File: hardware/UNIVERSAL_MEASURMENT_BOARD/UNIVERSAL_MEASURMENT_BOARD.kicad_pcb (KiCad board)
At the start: 2 copper layers, 68 parts, among them J10 2604-1104, J2 2606-1110_010-000, U1 ADS8863IDGS, U10 TPS54202HDDCR, U12 TPS54202HDDCR, U13 L7805ABD2T-TR, U14 ADM3055EBRIZ-RL, U15 TLV76133KVUR, U16 TLV76133KVUR, U2 LT3471EDD#PBF, U3 CD4067BM96, U4 PGA280AIPW, U5 CD4067BM96, U6 STM32G484RET3, U7 L7812ABD2T-TR, U8 MC7815BDTRKG, Y1 ECS-1612MV

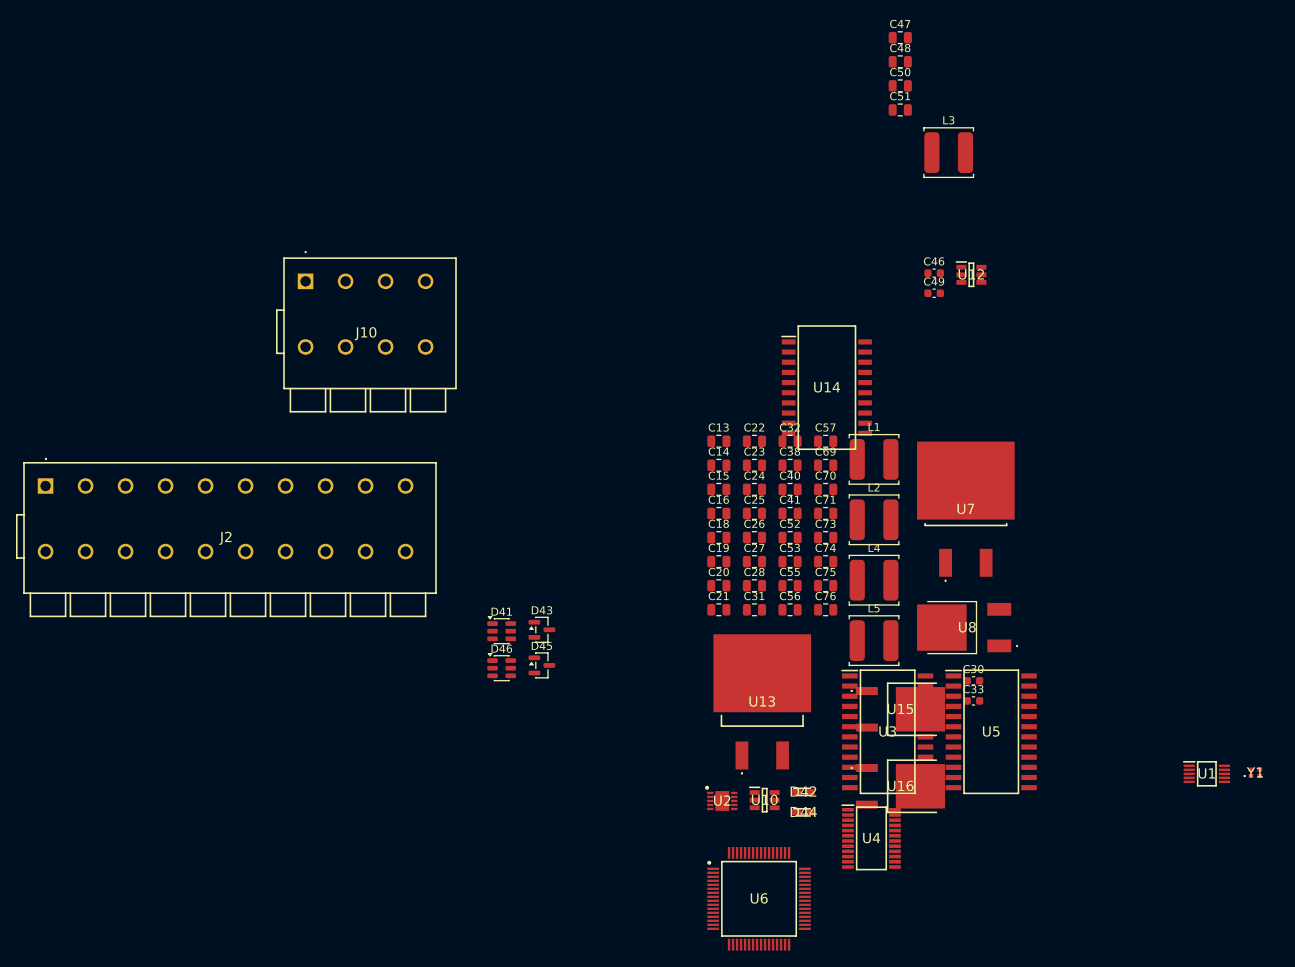
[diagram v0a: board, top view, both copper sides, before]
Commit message: final schematic review corrections
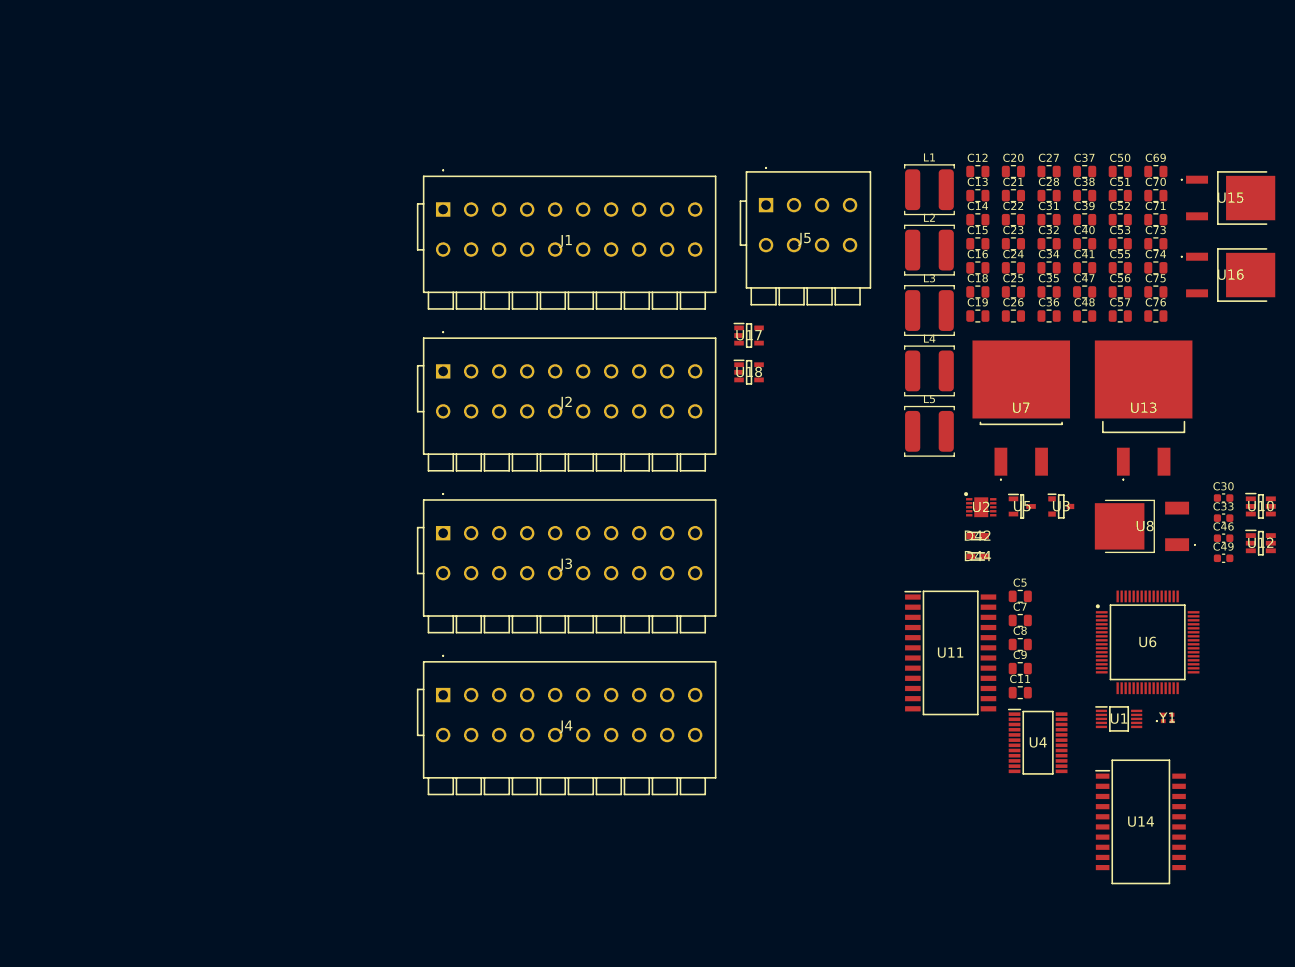
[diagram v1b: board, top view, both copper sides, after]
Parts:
- removed D41, D46: 3.6V/400W, Package_TO_SOT_SMD:SOT-23-6
- removed D43: BZX84C5V6, Package_TO_SOT_SMD:SOT-23
- removed D45: BZX84C3V6-E3-08, Package_TO_SOT_SMD:SOT-23
- removed J10: 2604-1104, 2604-1104:26041104
- added C11: 100nF, Capacitor_SMD:C_0805_2012Metric, F.Cu at (165.4, 110.4)
- added C12: 1uF, Capacitor_SMD:C_0805_2012Metric, F.Cu at (160.2, 45.3)
- added C34: 100nF, Capacitor_SMD:C_0805_2012Metric, F.Cu at (169.1, 57.3)
- added C35: 1uF, Capacitor_SMD:C_0805_2012Metric, F.Cu at (169.1, 60.3)
- added C36: 1uF, Capacitor_SMD:C_0805_2012Metric, F.Cu at (169.1, 63.4)
- added C37: 100nF, Capacitor_SMD:C_0805_2012Metric, F.Cu at (173.5, 45.3)
- added C39: 1uF, Capacitor_SMD:C_0805_2012Metric, F.Cu at (173.5, 51.3)
- added C5: 100nF, Capacitor_SMD:C_0805_2012Metric, F.Cu at (165.4, 98.4)
- added C7: 470nF, Capacitor_SMD:C_0805_2012Metric, F.Cu at (165.4, 101.4)
- added C8: 470nF, Capacitor_SMD:C_0805_2012Metric, F.Cu at (165.4, 104.4)
- added C9: 470nF, Capacitor_SMD:C_0805_2012Metric, F.Cu at (165.4, 107.4)
- added J1: 2606-1110_010-000, 2601-1110:26011110, F.Cu at (93.3, 50.0)
- added J3: 2606-1110_010-000, 2601-1110:26011110, F.Cu at (93.3, 90.5)
- added J4: 2606-1110_010-000, 2601-1110:26011110, F.Cu at (93.3, 110.7)
- added J5: 2604-1104, 2601-1104:26011104, F.Cu at (133.7, 49.5)
- added U11: CD4097BM, CD4097BM:SOIC127P1030X265-24N, F.Cu at (156.8, 105.5)
- added U17: ESDS304DBVR, ESDS304DBVR:SOT95P280X145-5N, F.Cu at (131.6, 65.8)
- added U18: ESDS304DBVR, ESDS304DBVR:SOT95P280X145-5N, F.Cu at (131.6, 70.4)
- J2: footprint 2604-1110:26041110 -> 2601-1110:26011110
- U3: value CD4067BM96 -> MAX6063AEUR+T; footprint CD4067BM96:SOIC127P1030X265-24N -> MAX6063AEUR+T:SOT95P229X119-3N
- U5: value CD4067BM96 -> ISL21010CFH315Z-TK; footprint CD4067BM96:SOIC127P1030X265-24N -> ISL21010CFH315Z-TK:SOT95P237X112-3N
- moved U15 76.1 mm to (191.9, 48.6)
- moved U16 76.1 mm to (191.9, 58.2)
- moved U10 72.1 mm to (195.5, 87.2)
- moved U14 67.0 mm to (180.5, 126.6)
- moved C21 63.5 mm to (164.6, 48.3)
- moved C20 63.5 mm to (164.6, 45.3)
- moved C27 61.1 mm to (169.1, 45.3)
- moved C31 61.1 mm to (169.1, 51.3)
- moved C28 61.1 mm to (169.1, 48.3)
- moved U13 60.2 mm to (180.9, 75.2)
- moved U6 58.2 mm to (181.4, 104.1)
- moved C52 57.3 mm to (177.9, 51.3)
- moved C53 57.3 mm to (177.9, 54.3)
- moved C55 57.3 mm to (177.9, 57.3)
- moved C56 57.3 mm to (177.9, 60.3)
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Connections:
- net +12VA renamed +12V0A
- net +15V renamed +15V0
- net +15VF renamed +15V0F
- net +18V renamed +18V0
- net +7V renamed +7V0
- net -18V renamed -18V0
- net /can/RX renamed /can/CAN_RX
- net /can/TX renamed /can/CAN_TX
- C16 pad 1: +15VA -> +15V0A
- C28 pad 2: -15VA -> -15V0A
- C57 pad 1: +5VA -> +5V0A
- U1 pad 1: Net-(U1-REF) -> +3V0A
- U13 pad 3: +5VA -> +5V0A
- U3 pad 1: Net-(U3-OUT) -> +5V0A
- U3 pad 2: /connectors/A8P -> +3V0A
- U3 pad 3: /connectors/A7P -> GND
- U4 pad 10: Net-(U4-INN1) -> /mux & pga/NS
- U4 pad 11: -15VA -> Net-(U4-VSN)
- U4 pad 13: +3.3VA -> Net-(U4-DVDD)
- U4 pad 3: unconnected-(U4-VOCM-Pad3) -> 1V5A
- U4 pad 4: +3.3VA -> Net-(U4-VSOP)
- U4 pad 6: +15VA -> Net-(U4-VSP)
- U4 pad 9: Net-(U3-OUT) -> /mux & pga/PS
- U5 pad 1: Net-(U4-INN1) -> +3V3A
- U5 pad 2: /connectors/A8N -> +1V5A
- U5 pad 3: /connectors/A7N -> GND
- U6 pad 28: unconnected-(U6-VREF+-Pad28) -> 3V0A
- U6 pad 30: /mcu & adc/UART_RX_PROG -> /connectors/UART_RX_PROG
- U6 pad 56: /mcu & adc/SWO -> /connectors/SWO
- U6 pad 7: /mcu & adc/NRST -> /connectors/NRST
- U6 pad 9: /mcu & adc/UART_TX_PROG -> /connectors/UART_TX_PROG
- U8 pad 3: +15VA -> +15V0A
